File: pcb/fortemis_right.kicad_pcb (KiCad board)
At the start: 2 copper layers, 124.2 x 100.8 mm, 26 parts

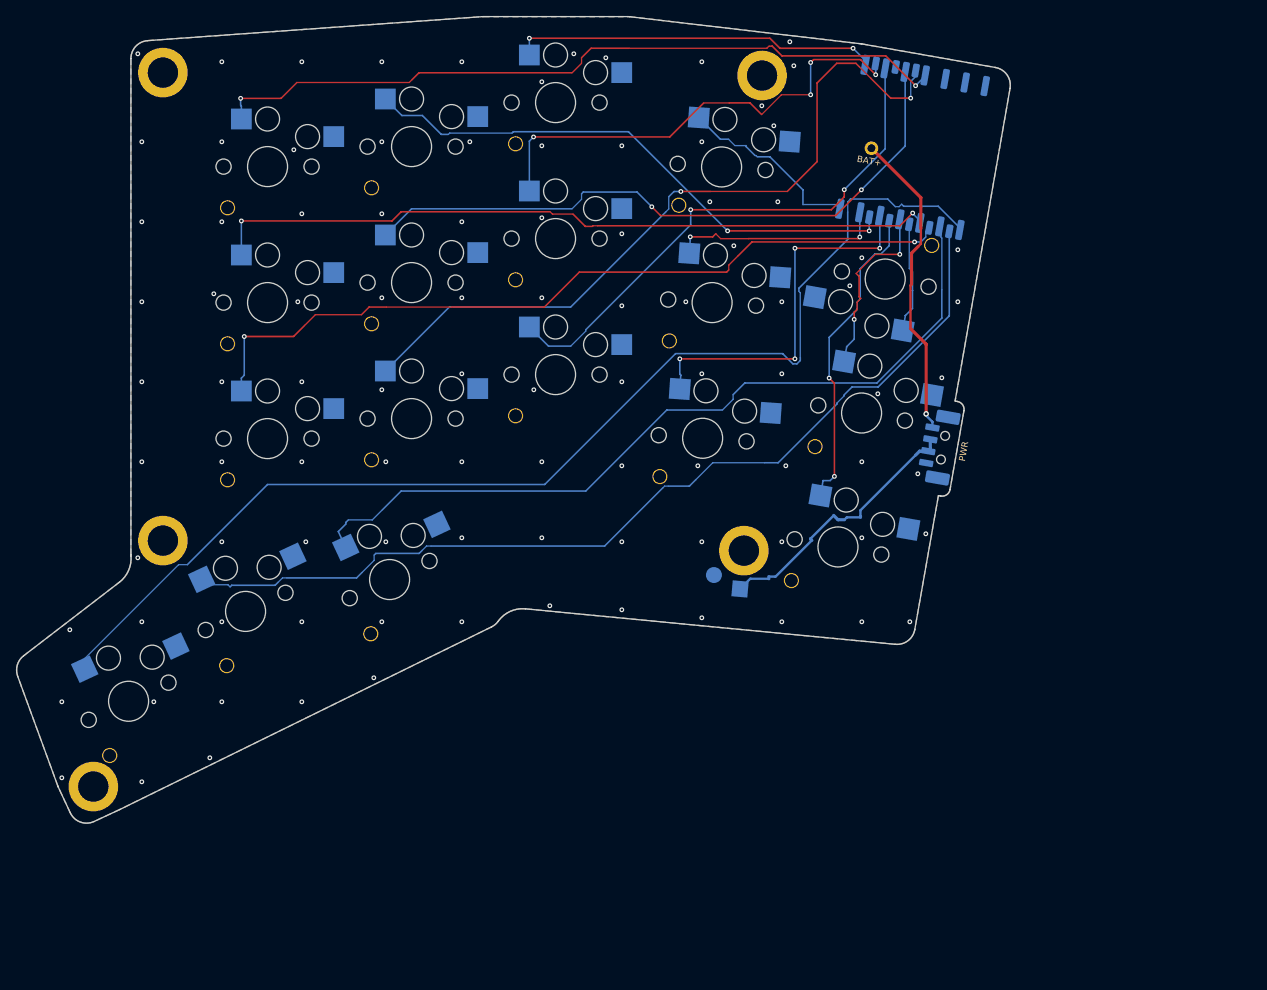
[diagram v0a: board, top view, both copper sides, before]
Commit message: Rebuild PCBs and fab files for the new thumbs
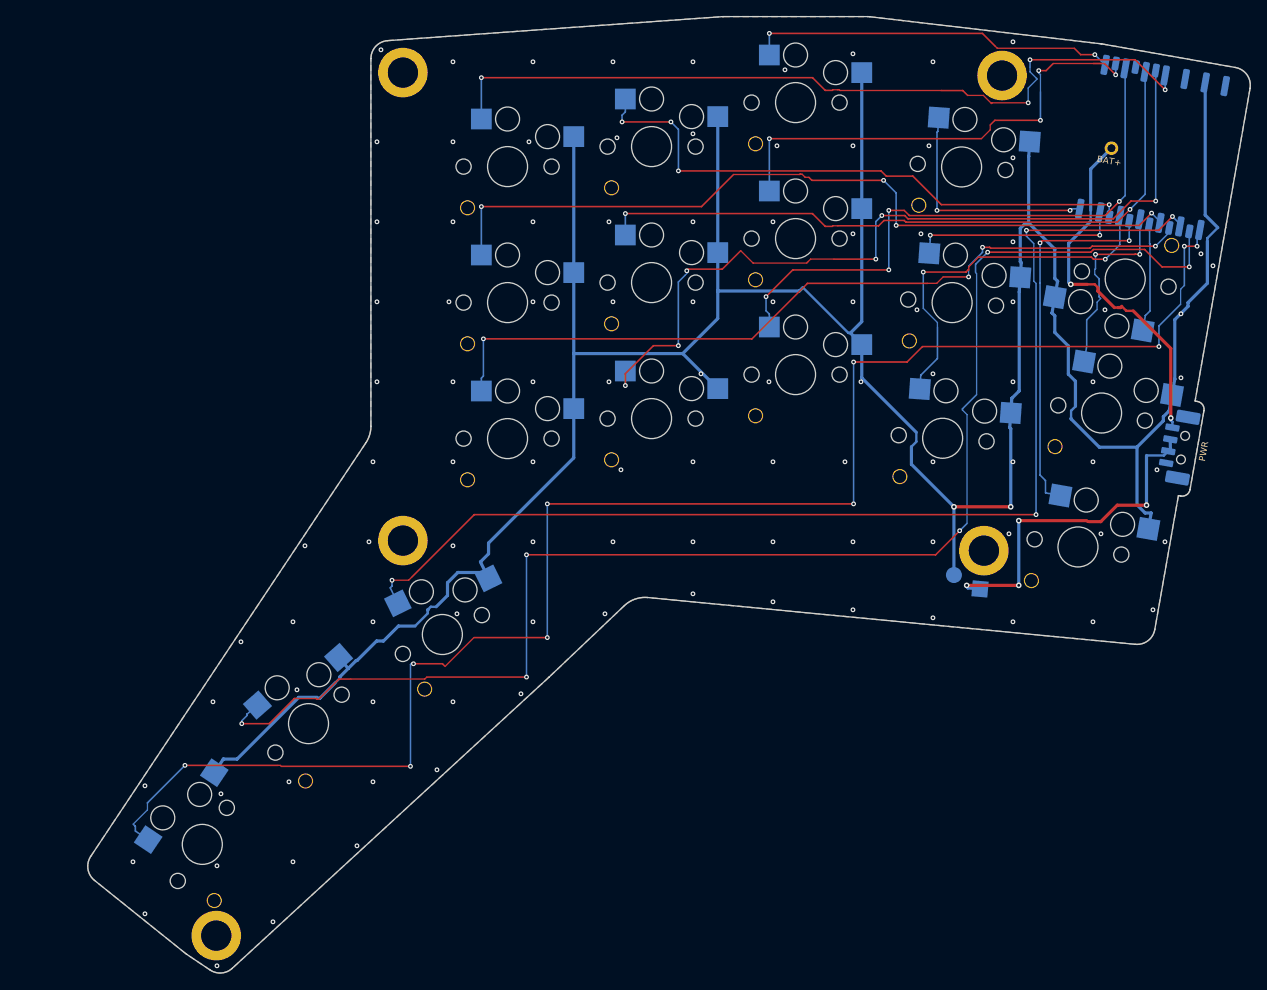
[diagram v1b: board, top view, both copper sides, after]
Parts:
- moved MCU1 30.0 mm to (271.9, -49.9)
- moved BT1 30.0 mm to (230.6, -0.69)
- moved NUT1 30.0 mm to (253.1, -58.9)
- moved NUT2 30.0 mm to (178.2, -59.3)
- moved NUT3 30.0 mm to (178.2, -0.79)
- moved NUT4 30.0 mm to (250.8, 0.47)
- moved PWR1 30.0 mm to (277.1, -12.2)
- moved S10 30.0 mm to (209.3, -33.0)
- moved S11 30.0 mm to (209.3, -50.0)
- moved S12 30.0 mm to (191.3, -13.5)
- moved S13 30.0 mm to (191.3, -30.5)
- moved S14 30.0 mm to (191.3, -47.5)
- moved S3 30.0 mm to (245.7, -13.6)
- moved S4 30.0 mm to (246.9, -30.5)
- moved S5 30.0 mm to (248.1, -47.5)
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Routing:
- net GND: track 0.00 -> 401.1 mm, vias 97 -> 106
- net D11: track 119.2 -> 179.5 mm, vias 0 -> 6
- net D0: track 146.1 -> 202.1 mm, vias 0 -> 10
- net D1: track 100.7 -> 143.7 mm, vias 0 -> 4
- net D19: track 93.8 -> 104.2 mm, vias 2 -> 6
- net BAT_RAW: track 33.7 -> 44.1 mm, vias 0 -> 4
- net D14: track 39.4 -> 47.2 mm
- net D10: track 93.9 -> 101.4 mm, vias 2 -> 4
- net D8: track 67.5 -> 74.9 mm, vias 2 -> 4
- net D2: track 91.8 -> 98.8 mm, vias 2 -> 4
- net BAT_P: track 39.2 -> 45.5 mm, vias 1 -> 2
- net D6: track 23.5 -> 29.6 mm, vias 0 -> 2
- net D9: track 81.7 -> 85.4 mm
- net D15: track 69.3 -> 72.8 mm, vias 2 -> 4
- net D3: track 22.8 -> 24.5 mm
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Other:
- board size 124.2 x 100.8 mm -> 145.3 x 119.6 mm
